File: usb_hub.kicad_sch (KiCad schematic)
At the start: 6 parts, among them J3 USB_C_Receptacle_USB2.0_16P, U2 SL2.1A

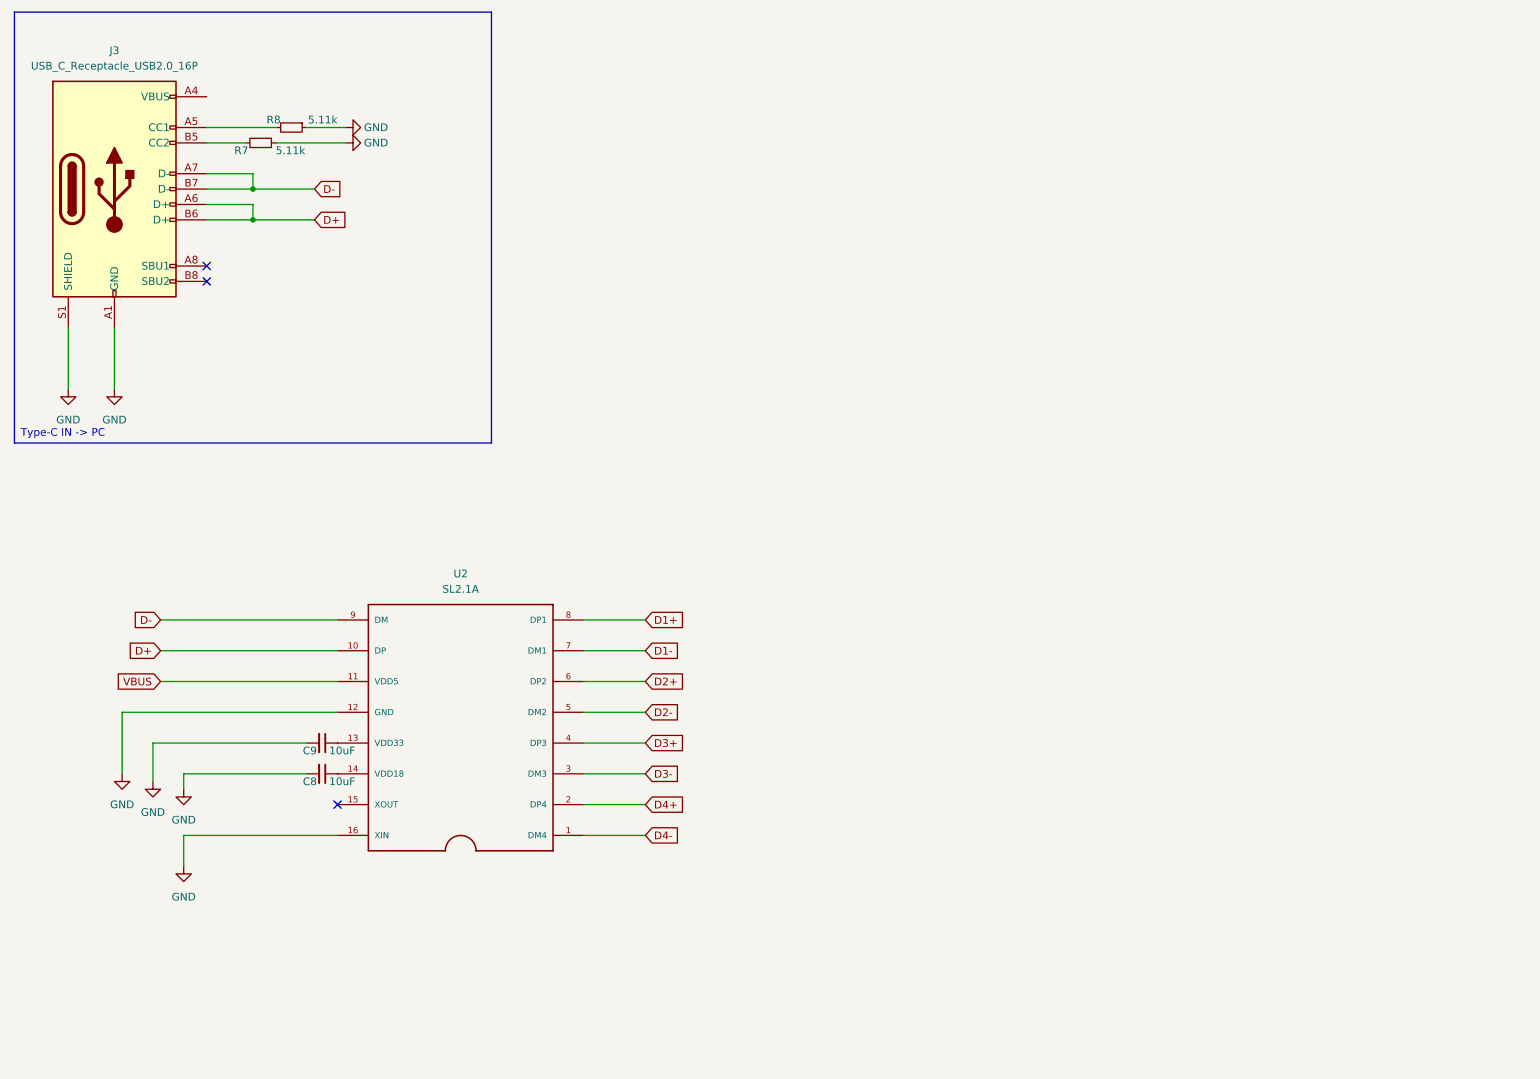
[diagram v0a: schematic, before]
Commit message: many things changed
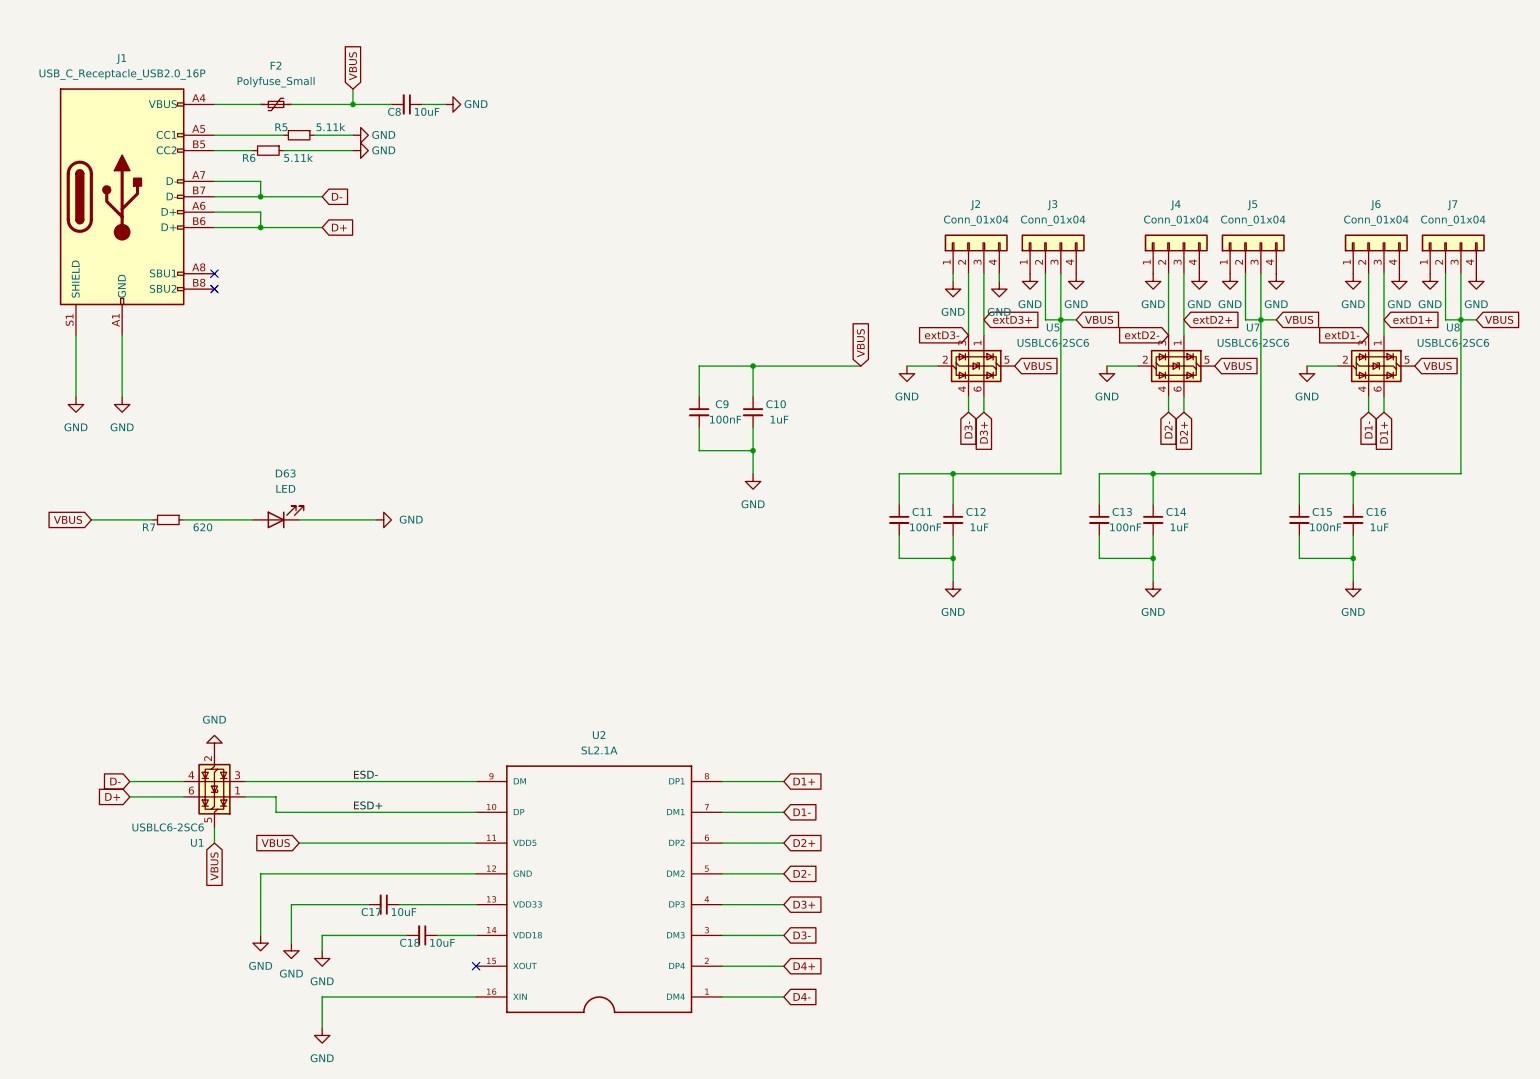
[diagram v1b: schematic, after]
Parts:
- added C10, C12, C14, C16: 1uF, Capacitor_SMD:C_0603_1608Metric, symbol Device:C_Small
- added C11, C13, C15, C9: 100nF, Capacitor_SMD:C_0603_1608Metric, symbol Device:C_Small
- added C8: 10uF, Capacitor_SMD:C_0603_1608Metric, symbol Device:C_Small
- added D63: LED, LED_SMD:LED_0805_2012Metric, symbol Device:LED
- added F2: Polyfuse_Small, Fuse:Fuse_1206_3216Metric, symbol Device:Polyfuse_Small
- added J2, J3, J4, J5, J6, J7: Conn_01x04, CustomFootprints:4_Pad_2.54_Exposed, symbol Connector_Generic:Conn_01x04
- added R7: 620, Resistor_SMD:R_0603_1608Metric, symbol Device:R_Small
- added U1, U5, U7, U8: USBLC6-2SC6, Package_TO_SOT_SMD:SOT-23-6, symbol Power_Protection:USBLC6-2SC6
- C17: renamed from C9; footprint (none) -> Capacitor_SMD:C_0603_1608Metric
- C18: renamed from C8; footprint (none) -> Capacitor_SMD:C_0603_1608Metric
- U2: MPN (none) -> C6798314
- renumbered J3 to J1, R8 to R5, R7 to R6
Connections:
- net D+: now also U1.6 (I/O1); no longer U2.10 (DP)
- net D-: now also U1.4 (I/O2); no longer U2.9 (DM)
- net D1+: now also U8.6 (I/O1)
- net D1-: now also U8.4 (I/O2)
- net D2+: now also U7.6 (I/O1)
- net D2-: now also U7.4 (I/O2)
- net D3+: now also U5.6 (I/O1)
- net D3-: now also U5.4 (I/O2)
- net GND: now also C10.2, C11.2, C12.2, C13.2, C14.2, C15.2, C16.2, C8.1, C9.2, D63.1 (K), J2.1 (Pin_1), J2.4 (Pin_4), J3.1 (Pin_1), J3.4 (Pin_4), J4.1 (Pin_1), J4.4 (Pin_4), J5.1 (Pin_1), J5.4 (Pin_4), J6.1 (Pin_1), J6.4 (Pin_4), J7.1 (Pin_1), J7.4 (Pin_4), U1.2 (GND), U5.2 (GND), U7.2 (GND), U8.2 (GND)
- net VBUS: now also C10.1, C11.1, C12.1, C13.1, C14.1, C15.1, C16.1, C8.2, C9.1, F2.2, J3.2 (Pin_2), J3.3 (Pin_3), J5.2 (Pin_2), J5.3 (Pin_3), J7.2 (Pin_2), J7.3 (Pin_3), R7.2, U1.5 (VBUS), U5.5 (VBUS), U7.5 (VBUS), U8.5 (VBUS)
- net at J1.A4 (VBUS), J1.A9 (VBUS), J1.B4 (VBUS)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: now also F2.1
- new net: D63.2 (A), R7.1
- new net ESD+: U1.1 (I/O1), U2.10 (DP)
- new net ESD-: U1.3 (I/O2), U2.9 (DM)
- new net extD1+: J6.3 (Pin_3), U8.1 (I/O1)
- new net extD1-: J6.2 (Pin_2), U8.3 (I/O2)
- new net extD2+: J4.3 (Pin_3), U7.1 (I/O1)
- new net extD2-: J4.2 (Pin_2), U7.3 (I/O2)
- new net extD3+: J2.3 (Pin_3), U5.1 (I/O1)
- new net extD3-: J2.2 (Pin_2), U5.3 (I/O2)
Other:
- moved on the sheet: C17, C18, J1, R5, R6, U2
